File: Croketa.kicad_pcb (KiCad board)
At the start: 2 copper layers, 17.8 x 33 mm, 25 parts, among them J1 USB_B_Micro, J2 Conn_02x02_Odd_Even, P1 Digital, P4 Analog, SW1 SW_DPST_x2, U1 AP2112K-3.3TRG1, U2 ATSAMD21E18A-AF

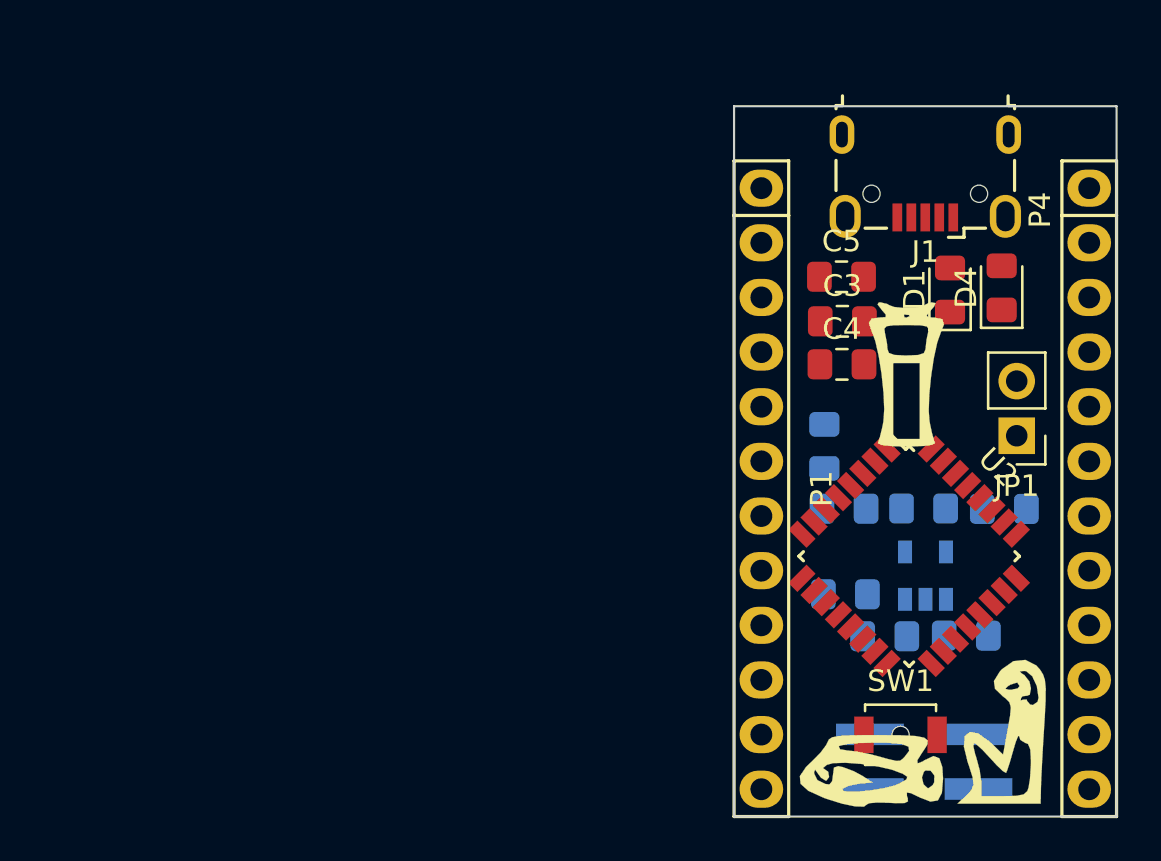
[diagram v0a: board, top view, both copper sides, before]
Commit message: New pcb's Bast
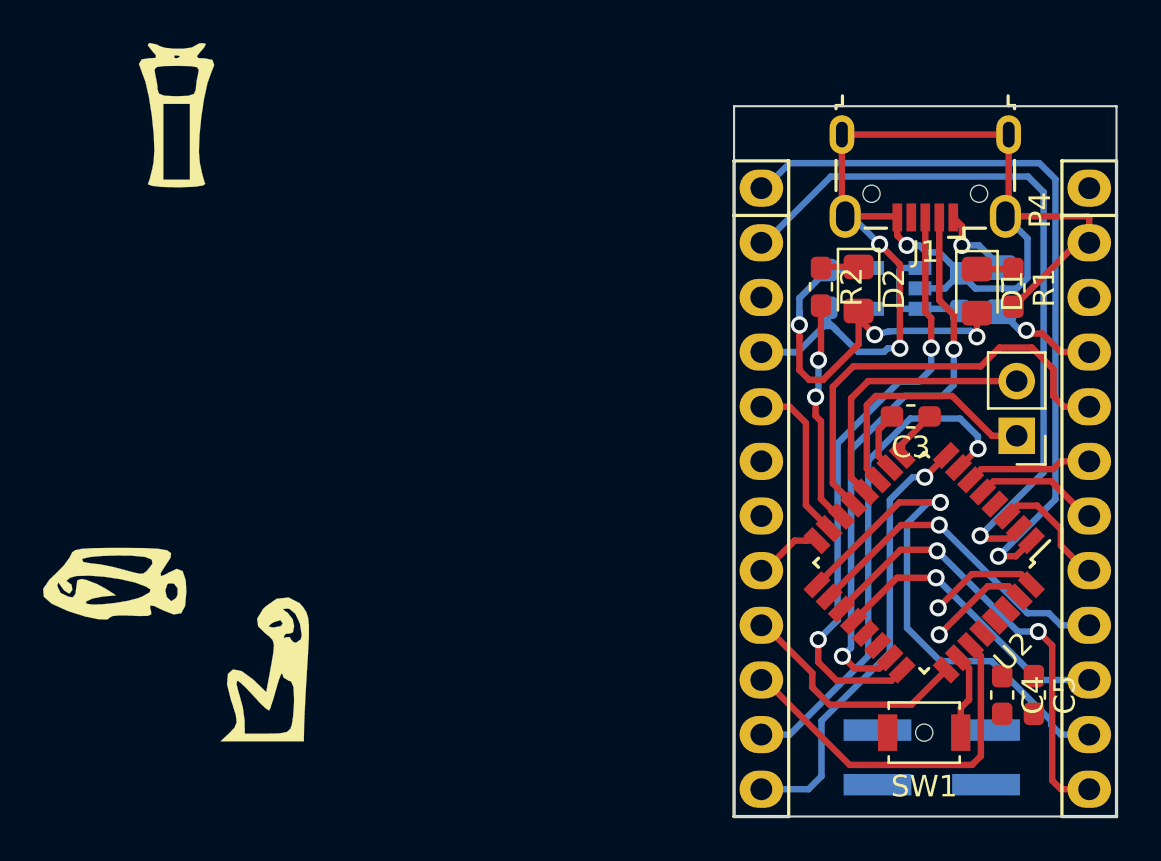
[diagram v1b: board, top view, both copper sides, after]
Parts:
- removed D4: LED, LED_SMD:LED_0805_2012Metric_Pad1.15x1.40mm_HandSolder
- removed R3, R4: 330, Resistor_SMD:R_0805_2012Metric_Pad1.15x1.40mm_HandSolder
- added D2: LED, LED_SMD:LED_0805_2012Metric_Pad1.15x1.40mm_HandSolder, F.Cu at (142.9, 89.8)
- C1, C2, C3, C4, C5: footprint Capacitor_SMD:C_0805_2012Metric_Pad1.15x1.40mm_HandSolder -> Capacitor_SMD:C_0603_1608Metric_Pad1.05x0.95mm_HandSolder
- P2: renamed from JP1; value Jumper_NC_Small -> ADC
- R1, R2: footprint Resistor_SMD:R_0805_2012Metric_Pad1.15x1.40mm_HandSolder -> Resistor_SMD:R_0603_1608Metric_Pad1.05x0.95mm_HandSolder; moved to F.Cu
- moved G*** 52.2 mm to (94.0, 90.1)
- moved REF*** 51.4 mm to (94.8, 84.2)
- moved G*** 36.2 mm to (108.3, 103.4)
- moved G*** 36.0 mm to (111.2, 81.7)
- moved G*** 34.4 mm to (115.3, 107.5)
- moved C5 21.4 mm to (151.1, 108.7), turned to 270 degrees
- moved C2 17.4 mm to (141.5, 89.8), turned to 270 degrees
- moved C4 17.1 mm to (149.6, 108.7), turned to 270 degrees
- moved C1 16.4 mm to (147.7, 89.9), turned to 90 degrees
- moved F1 15.9 mm to (149.6, 89.8), turned to 90 degrees
- moved U1 13.4 mm to (144.7, 89.8), turned to 180 degrees
- moved R2 13.4 mm to (141.2, 89.7), turned to 270 degrees
- moved R1 11.1 mm to (150.2, 89.7), turned to 270 degrees
- moved C3 5.45 mm to (145.4, 95.7), turned to 180 degrees
- moved D1 1.25 mm to (148.4, 89.9), turned to 270 degrees
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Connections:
- P2 pad 1: Net-(JP1-Pad1) -> /SDA
- P2 pad 2: GND -> /SCL
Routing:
- net GND: track 0.00 -> 62.8 mm, vias 0 -> 3
- net /1(Tx): track 0.00 -> 34.9 mm, vias 0 -> 1
- net /0(Rx): track 0.00 -> 34.0 mm, vias 0 -> 1
- net /D+: track 0.00 -> 28.0 mm, vias 0 -> 2
- net /D-: track 0.00 -> 27.3 mm, vias 0 -> 2
- net /11(**/MOSI): track 0.00 -> 24.8 mm, vias 0 -> 1
- net /8: track 0.00 -> 23.7 mm, vias 0 -> 1
- net /10(**/SS): track 0.00 -> 21.0 mm, vias 0 -> 2
- net +3V3: track 0.00 -> 20.8 mm, vias 0 -> 3
- net /9(**): track 0.00 -> 20.7 mm, vias 0 -> 1
- net /A3: track 0.00 -> 20.4 mm
- net /7: track 0.00 -> 17.3 mm
- net /13(SCK): track 0.00 -> 15.4 mm, vias 0 -> 1
- net /12(MISO): track 0.00 -> 13.8 mm, vias 0 -> 1
- net /SCL: track 0.00 -> 12.7 mm
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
